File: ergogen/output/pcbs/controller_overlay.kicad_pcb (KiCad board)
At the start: 2 copper layers, 19.7 x 60.1 mm, 2 parts

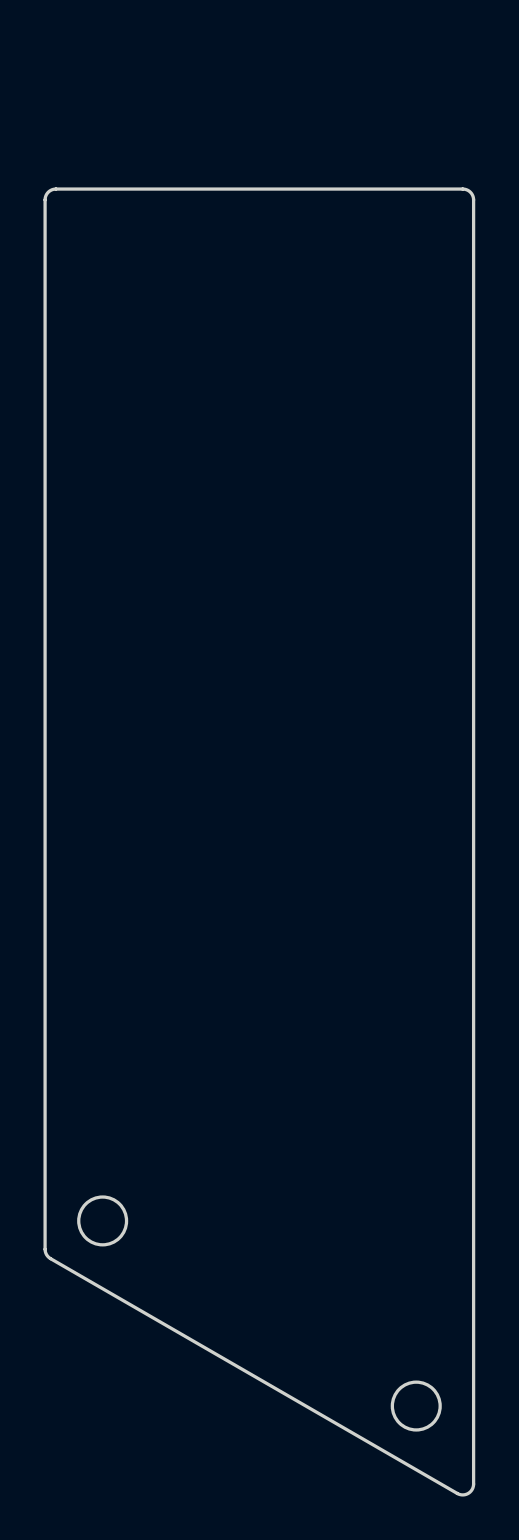
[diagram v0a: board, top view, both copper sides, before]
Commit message: Checkpoint
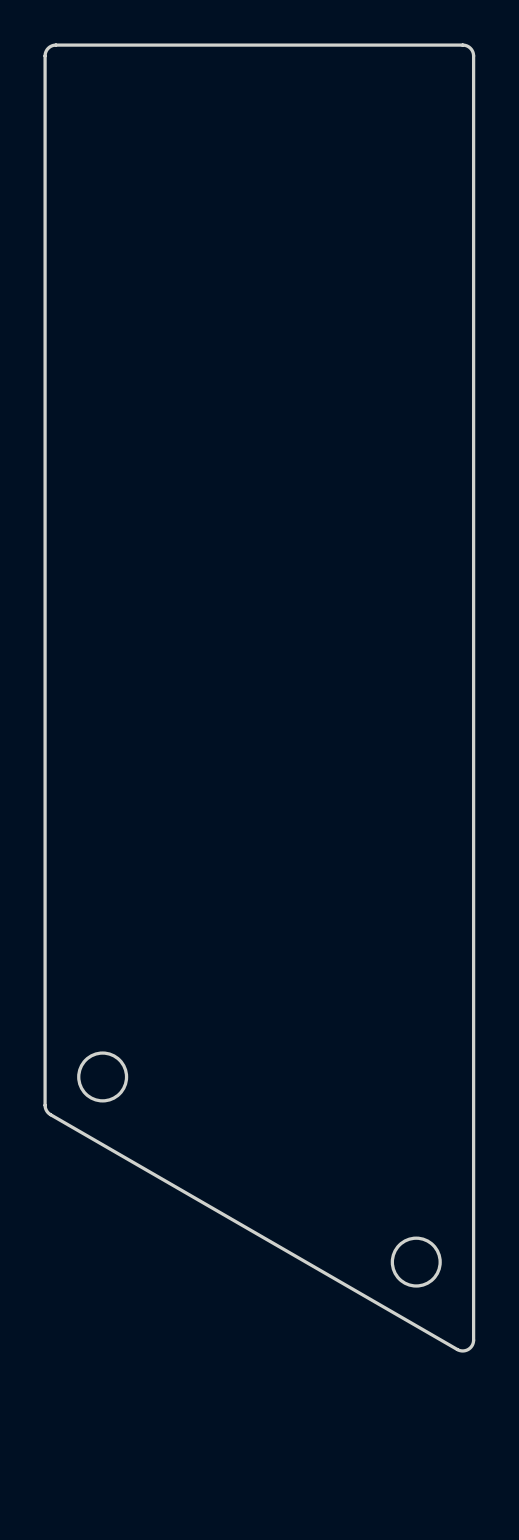
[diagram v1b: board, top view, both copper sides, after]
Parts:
- moved MH1 6.62 mm to (207.8, 93.9)
- moved MH2 6.62 mm to (222.2, 102.4)
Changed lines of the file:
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@@
   )
   (module "ceoloide:mounting_hole_npth" (layer F.Cu)
-      (at 207.762 100.476 0)
+      (at 207.762 93.851 0)
       (fp_text reference "MH1" (at 0 2.55 0) (layer F.SilkS) hide (effects (font (size 1 1) (thickness 0.15))))
       (pad "" np_thru_hole circle (at 0 0 0) (size 2.2 2.2) (drill 2.2) (layers *.Cu *.Mask))
   )
   (module "ceoloide:mounting_hole_npth" (layer F.Cu)
-      (at 222.194 108.995 0)
+      (at 222.194 102.37 0)
       (fp_text reference "MH2" (at 0 2.55 0) (layer F.SilkS) hide (effects (font (size 1 1) (thickness 0.15))))
       (pad "" np_thru_hole circle (at 0 0 0) (size 2.2 2.2) (drill 2.2) (layers *.Cu *.Mask))
   )
-            (gr_line (start 205.113 101.77697755907997) (end 205.113 53.49) (angle 90) (layer Edge.Cuts) (width 0.15))
-(gr_line (start 205.613 52.99) (end 224.333 52.99) (angle 90) (layer Edge.Cuts) (width 0.15))
-(gr_line (start 224.833 53.49) (end 224.833 112.58497459811554) (angle 90) (layer Edge.Cuts) (width 0.15))
-(gr_line (start 224.08299999999997 113.01798729811554) (end 205.36299999999997 102.20999025907994) (angle 90) (layer Edge.Cuts) (width 0.15))
-(gr_arc (start 205.613 53.49) (end 205.613 52.99) (angle -90) (layer Edge.Cuts) (width 0.15))
-(gr_arc (start 224.333 53.49) (end 224.833 53.49) (angle -90) (layer Edge.Cuts) (width 0.15))
-(gr_arc (start 224.333 112.58497459811554) (end 224.083 113.01798729811554) (angle -120.00000010841867) (layer Edge.Cuts) (width 0.15))
-(gr_arc (start 205.613 101.77697755907997) (end 205.113 101.77697755907997) (angle -59.999999891579705) (layer Edge.Cuts) (width 0.15))
-(gr_circle (center 207.762 100.476) (end 208.862 100.476) (layer Edge.Cuts) (width 0.15))
-(gr_circle (center 222.194 108.995) (end 223.29399999999998 108.995) (layer Edge.Cuts) (width 0.15))
+            (gr_line (start 205.113 95.15197755907997) (end 205.113 46.865) (angle 90) (layer Edge.Cuts) (width 0.15))
+(gr_line (start 205.613 46.365) (end 224.333 46.365) (angle 90) (layer Edge.Cuts) (width 0.15))
+(gr_line (start 224.833 46.865) (end 224.833 105.95997459811554) (angle 90) (layer Edge.Cuts) (width 0.15))
+(gr_line (start 224.08299999999997 106.39298729811554) (end 205.36299999999997 95.58499025907994) (angle 90) (layer Edge.Cuts) (width 0.15))
+(gr_arc (start 205.613 46.865) (end 205.613 46.365) (angle -90) (layer Edge.Cuts) (width 0.15))
+(gr_arc (start 224.333 46.865) (end 224.833 46.865) (angle -90) (layer Edge.Cuts) (width 0.15))
+(gr_arc (start 224.333 105.95997459811554) (end 224.083 106.39298729811554) (angle -120.00000010841867) (layer Edge.Cuts) (width 0.15))
+(gr_arc (start 205.613 95.15197755907997) (end 205.113 95.15197755907997) (angle -59.999999891579705) (layer Edge.Cuts) (width 0.15))
+(gr_circle (center 207.762 93.851) (end 208.862 93.851) (layer Edge.Cuts) (width 0.15))
+(gr_circle (center 222.194 102.37) (end 223.29399999999998 102.37) (layer Edge.Cuts) (width 0.15))
 )
